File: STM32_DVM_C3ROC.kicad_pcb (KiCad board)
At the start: 4 copper layers, 85.2 x 56 mm, 170 parts, among them IC2 MCP6002, IC3 MCP6002, IC4 MCP6002, J1 40HAT, J2 USB_B_Micro, Q1 Crystal_GND24, SW1 SW_Push, T1 MMUN2214, T2 MMUN2214, T3 MMUN2214, T4 MMUN2214, U1 STM32F446RETx, U2 USBLC6-2SC6, U3 USBLC6-2SC6, U4 USBLC6-2SC6, U5 TPS54360DDA, X1 IQXO-70, X2 To Radio

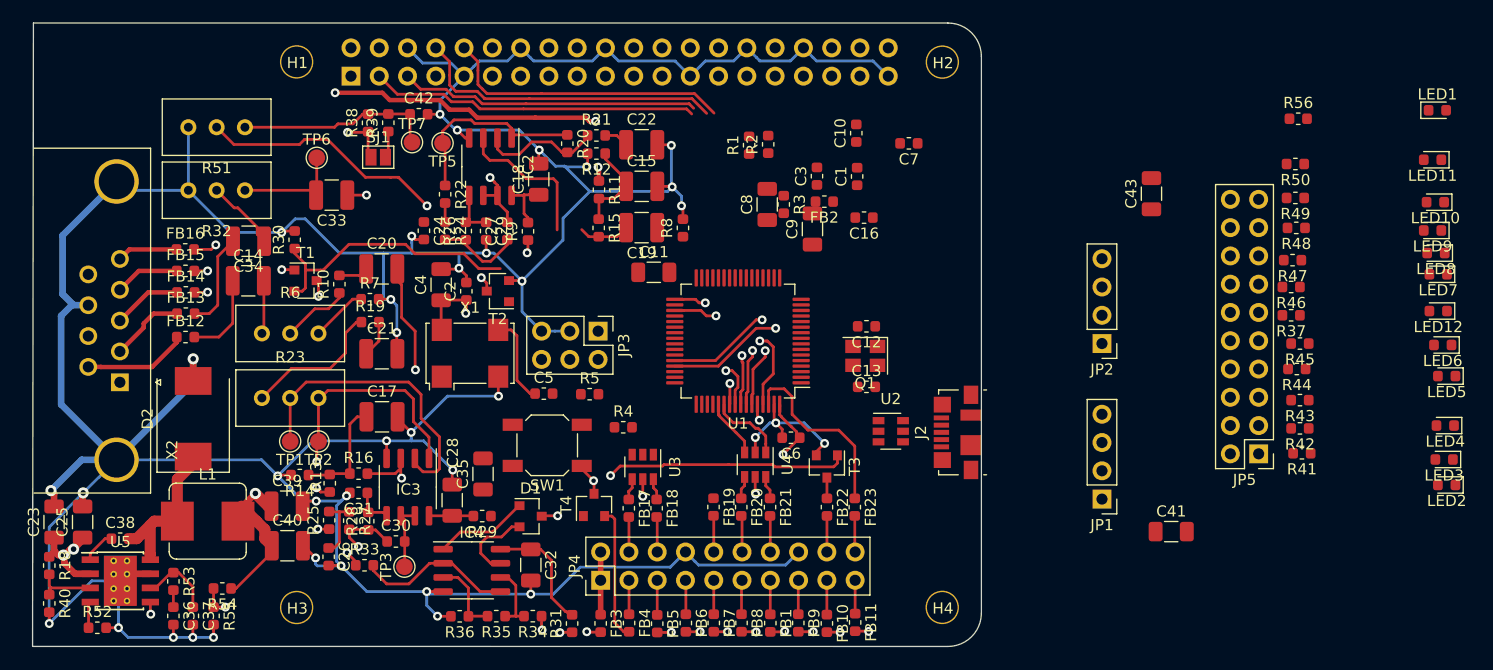
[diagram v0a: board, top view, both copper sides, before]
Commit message: Layout fertig für review
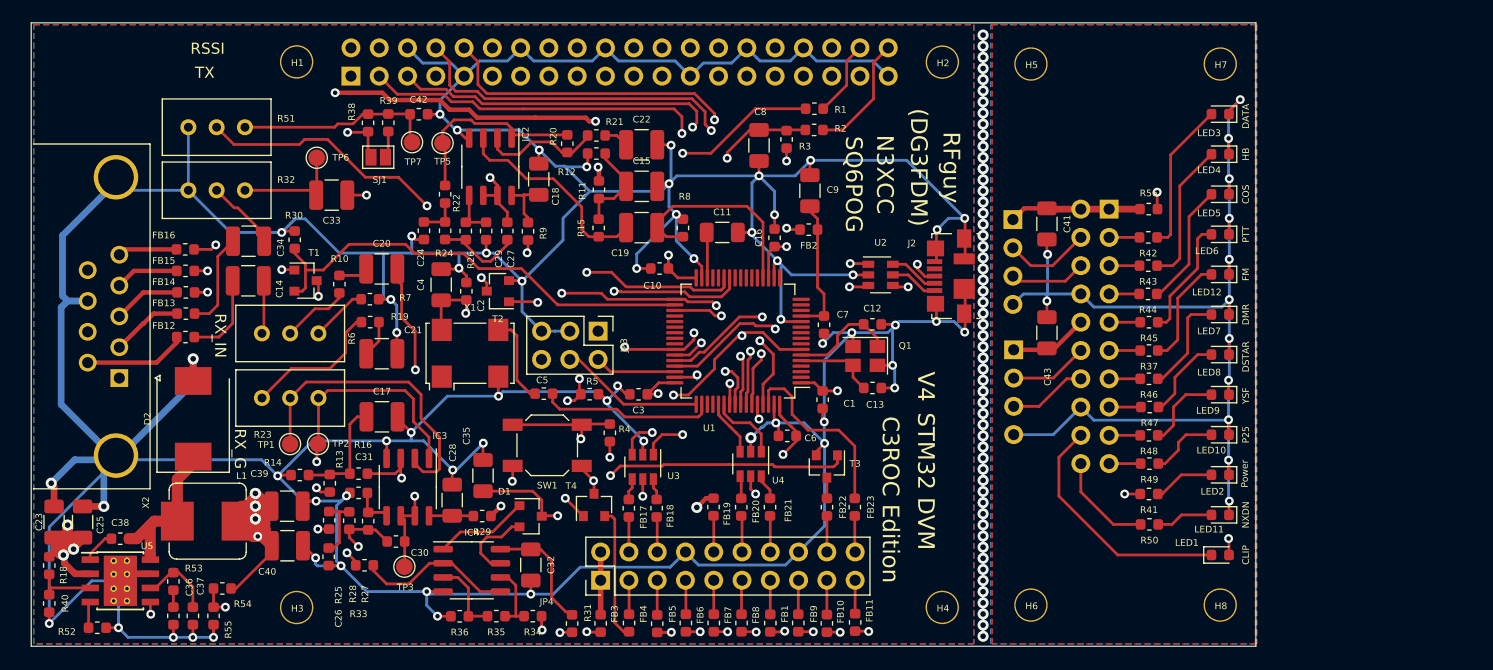
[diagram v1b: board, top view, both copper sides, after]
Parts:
- added H5: 3mm, project_footprints:NPTH_3mm_ID, F.Cu at (148.0, 64.5)
- added H6: 3mm, project_footprints:NPTH_3mm_ID, F.Cu at (148.0, 113.1)
- added H7: 3mm, project_footprints:NPTH_3mm_ID, F.Cu at (165.0, 64.5)
- added H8: 3mm, project_footprints:NPTH_3mm_ID, F.Cu at (165.0, 113.1)
- JP1, JP2, JP5: moved to B.Cu
- moved LED1 44.5 mm to (165.0, 108.6)
- moved LED11 37.2 mm to (165.0, 105.0)
- moved LED3 37.0 mm to (165.0, 69.0)
- moved R50 34.9 mm to (158.6, 105.9)
- moved LED4 31.7 mm to (165.0, 72.6)
- moved C41 29.8 mm to (149.4, 78.9), turned to 270 degrees
- moved LED10 28.5 mm to (165.0, 97.8)
- moved R49 27.2 mm to (158.6, 100.4)
- moved JP1 26.4 mm to (146.4, 78.5)
- moved LED5 26.1 mm to (165.0, 76.2)
- moved JP5 25.8 mm to (155.0, 77.5)
- moved C3 25.3 mm to (112.8, 94.2), turned to 180 degrees
- moved LED9 24.1 mm to (165.0, 94.2)
- moved R48 22.9 mm to (158.6, 97.9)
- moved LED6 22.3 mm to (165.0, 79.8)
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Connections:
- J1 pad 11: Net-(J1-Pad11) -> (no net)
- J1 pad 12: Net-(J1-Pad12) -> (no net)
- J1 pad 13: Net-(J1-Pad13) -> (no net)
- J1 pad 15: Net-(J1-Pad15) -> (no net)
- J1 pad 16: Net-(J1-Pad16) -> (no net)
- J1 pad 18: Net-(J1-Pad18) -> (no net)
- J1 pad 19: Net-(J1-Pad19) -> (no net)
- J1 pad 21: Net-(J1-Pad21) -> (no net)
- J1 pad 22: Net-(J1-Pad22) -> (no net)
- J1 pad 23: Net-(J1-Pad23) -> (no net)
- J1 pad 24: Net-(J1-Pad24) -> (no net)
- J1 pad 26: Net-(J1-Pad26) -> (no net)
- J1 pad 27: Net-(J1-Pad27) -> (no net)
- J1 pad 28: Net-(J1-Pad28) -> (no net)
- J1 pad 29: Net-(J1-Pad29) -> (no net)
- J1 pad 31: Net-(J1-Pad31) -> (no net)
- J1 pad 32: Net-(J1-Pad32) -> (no net)
- J1 pad 33: Net-(J1-Pad33) -> (no net)
- J1 pad 35: Net-(J1-Pad35) -> (no net)
- J1 pad 36: Net-(J1-Pad36) -> (no net)
- J1 pad 37: Net-(J1-Pad37) -> (no net)
- J1 pad 7: Net-(J1-Pad7) -> (no net)
- J2 pad 4: Net-(J2-Pad4) -> (no net)
- U1 pad 10: Net-(U1-Pad10) -> (no net)
- U1 pad 11: Net-(U1-Pad11) -> (no net)
- U1 pad 14: Net-(U1-Pad14) -> (no net)
- U1 pad 15: Net-(U1-Pad15) -> (no net)
- U1 pad 16: Net-(U1-Pad16) -> (no net)
- U1 pad 17: Net-(U1-Pad17) -> (no net)
- U1 pad 2: Net-(U1-Pad2) -> (no net)
- U1 pad 21: Net-(U1-Pad21) -> (no net)
- U1 pad 22: Net-(U1-Pad22) -> (no net)
- U1 pad 23: Net-(U1-Pad23) -> (no net)
- U1 pad 24: Net-(U1-Pad24) -> (no net)
- U1 pad 25: Net-(U1-Pad25) -> (no net)
- U1 pad 28: BOOT1 -> (no net)
- U1 pad 29: Net-(U1-Pad29) -> (no net)
- U1 pad 3: Net-(U1-Pad3) -> (no net)
- U1 pad 36: Net-(U1-Pad36) -> (no net)
- U1 pad 37: Net-(U1-Pad37) -> (no net)
- U1 pad 38: Net-(U1-Pad38) -> (no net)
- U1 pad 39: Net-(U1-Pad39) -> (no net)
- U1 pad 4: Net-(U1-Pad4) -> (no net)
- U1 pad 40: Net-(U1-Pad40) -> (no net)
- U1 pad 41: Net-(U1-Pad41) -> (no net)
- U1 pad 51: Net-(U1-Pad51) -> (no net)
- U1 pad 52: Net-(U1-Pad52) -> (no net)
- U1 pad 8: Net-(U1-Pad8) -> (no net)
- U1 pad 9: Net-(U1-Pad9) -> (no net)
- X1 pad 1: Net-(X1-Pad1) -> (no net)
- X2 pad 1: Net-(X2-Pad1) -> (no net)
- X2 pad 7: Net-(X2-Pad7) -> (no net)
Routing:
- net GND: track 421.7 -> 599.3 mm, vias 37 -> 61
- net +3V3: track 167.4 -> 284.7 mm, vias 11 -> 18
- net GNDA: track 0.00 -> 100.5 mm, vias 0 -> 13
- net +5V: track 110.4 -> 167.2 mm, vias 4 -> 9
- net BOOT0: track 0.00 -> 55.9 mm, vias 0 -> 4
- net TXD_HOST: track 26.1 -> 80.7 mm, vias 0 -> 4
- net NRST: track 0.00 -> 54.1 mm, vias 0 -> 3
- net RXA: track 6.00 -> 53.9 mm, vias 0 -> 2
- net +3.3VA: track 0.00 -> 41.1 mm, vias 0 -> 1
- net Net-(LED1-Pad2): track 0.00 -> 37.5 mm, vias 0 -> 2
- net SCL: track 26.9 -> 61.9 mm, vias 0 -> 2
- net SDA: track 29.5 -> 62.9 mm, vias 0 -> 2
- net RXD_HOST: track 28.0 -> 52.3 mm, vias 0 -> 2
- net Net-(JP5-Pad18): track 0.00 -> 22.2 mm
- net TXA: track 0.00 -> 18.8 mm
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- added copper zone on In2.Cu, net +3.3VA
- added copper zone on In2.Cu, net +3V3
- added copper zone on In2.Cu, net +5V
- added copper zone on In2.Cu, net +BATT
- added copper zone on B.Cu, net GND
- added copper zone on F.Cu, net GND
- added copper zone on B.Cu, net GNDA
- added copper zone on F.Cu, net GNDA
- removed copper zone on In2.Cu, net INHIBIT
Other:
- board size 85.2 x 56 mm -> 110 x 56 mm
- board text added: "(DG3FDM)"
- board text added: "C3ROC Edition"
- board text added: "CLIP"
- board text added: "COS"
- board text added: "DATA"
- board text added: "DMR"
- board text added: "DSTAR"
- board text added: "FM"
- board text added: "HB"
- board text added: "N3XCC"
- board text added: "NXDN"
- board text added: "P25"
- board text added: "PTT"
- board text added: "Power"
- board text added: "RFguy"
- board text added: "RSSI"
- board text added: "RX_G"
- board text added: "RX_IN"
- board text added: "SQ6POG"
- board text added: "STM32 DVM"
- board text added: "TX"
- board text added: "V4"
- board text added: "YSF"
